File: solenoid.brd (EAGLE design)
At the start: 35.6 x 30.5 mm, 40 parts, among them Y1 ECS-80-S-4X

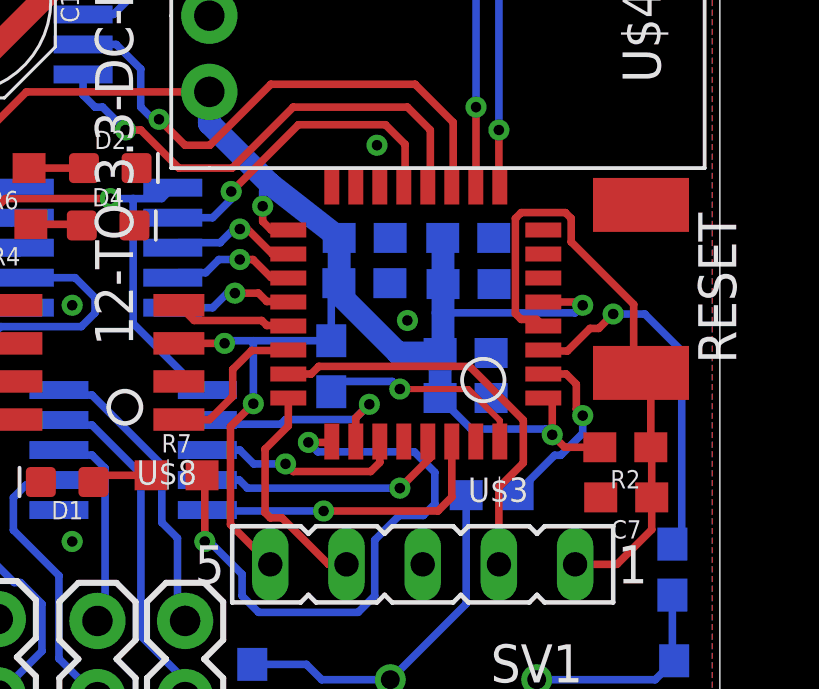
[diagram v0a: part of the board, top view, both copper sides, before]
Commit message: Update solenoid.brd
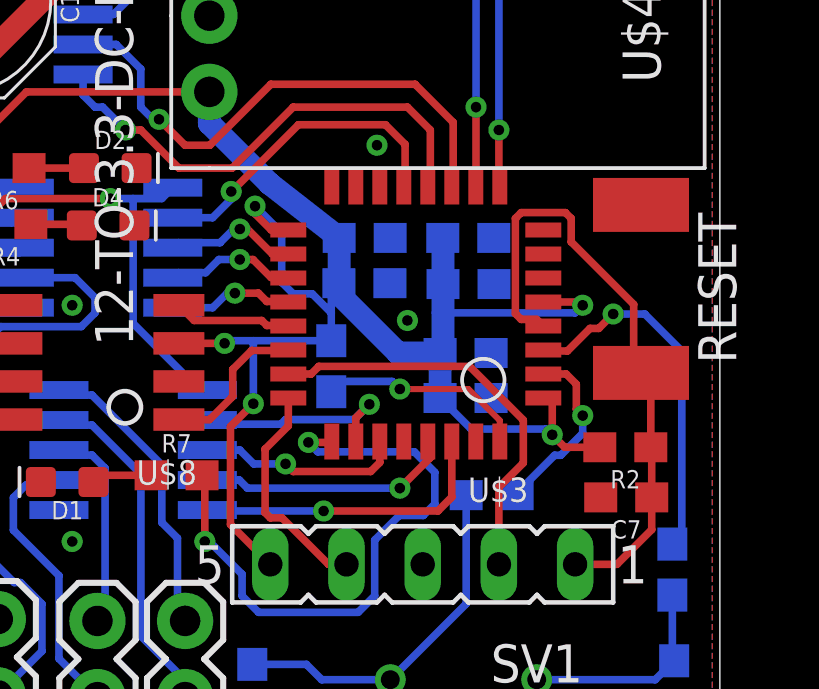
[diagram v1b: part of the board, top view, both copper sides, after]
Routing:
- net +3V3: track 59.1 -> 63.3 mm
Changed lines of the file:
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@@
 <wire x1="29.972" y1="12.148" x2="29.674" y2="12.148" width="0.254" layer="1"/>
 <wire x1="29.972" y1="10.922" x2="29.972" y2="12.148" width="0.254" layer="1"/>
-<wire x1="20.558" y1="19.288" x2="20.32" y2="19.05" width="0.254" layer="16"/>
-<wire x1="20.32" y1="19.05" x2="20.32" y2="18.542" width="0.254" layer="16"/>
-<via x="20.32" y="18.542" extent="1-16" drill="0.35"/>
-<wire x1="20.32" y1="18.542" x2="20.32" y2="18.034" width="0.254" layer="1"/>
-<wire x1="20.32" y1="18.034" x2="20.606" y2="17.748" width="0.254" layer="1"/>
+<via x="20.066" y="18.542" extent="1-16" drill="0.35"/>
+<wire x1="20.066" y1="18.542" x2="20.066" y2="18.288" width="0.254" layer="1"/>
+<wire x1="20.066" y1="18.288" x2="20.606" y2="17.748" width="0.254" layer="1"/>
 <wire x1="20.606" y1="17.748" x2="21.174" y2="17.748" width="0.254" layer="1"/>
 <wire x1="31.558" y1="10.506" x2="30.388" y2="10.506" width="0.254" layer="1"/>
@@
 <via x="20.0084" y="11.95728125" extent="1-16" drill="0.35"/>
 <wire x1="22.86" y1="15.976" x2="22.606" y2="15.722" width="0.254" layer="16"/>
-<wire x1="22.606" y1="15.722" x2="22.606" y2="14.058" width="0.254" layer="16"/>
+<wire x1="22.606" y1="15.722" x2="22.606" y2="14.986" width="0.254" layer="16"/>
+<wire x1="22.606" y1="14.058" x2="22.606" y2="14.986" width="0.254" layer="16"/>
 <wire x1="22.606" y1="14.058" x2="20.0084" y2="14.058" width="0.254" layer="16"/>
 <wire x1="20.0084" y1="14.058" x2="19.138" y2="14.058" width="0.254" layer="16"/>
@@
 <wire x1="10.834" y1="20.74" x2="12.446" y2="22.352" width="0.254" layer="1"/>
 <wire x1="12.446" y1="22.352" x2="18.542" y2="22.352" width="0.254" layer="1"/>
+<wire x1="22.606" y1="14.986" x2="21.971" y2="15.621" width="0.254" layer="16"/>
+<wire x1="21.971" y1="15.621" x2="21.336" y2="15.621" width="0.254" layer="16"/>
+<wire x1="21.336" y1="15.621" x2="20.955" y2="16.002" width="0.254" layer="16"/>
+<wire x1="20.955" y1="16.002" x2="20.955" y2="17.653" width="0.254" layer="16"/>
+<wire x1="20.955" y1="17.653" x2="20.066" y2="18.542" width="0.254" layer="16"/>
 </signal>
 <signal name="GPIO1">
@@
 <wire x1="33.258" y1="10.506" x2="33.288" y2="10.476" width="0.254" layer="1"/>
 <wire x1="33.288" y1="10.476" x2="33.288" y2="8.836" width="0.254" layer="1"/>
-<wire x1="33.288" y1="8.836" x2="33.288" y2="8.58286875" width="0.254" layer="1"/>
 <wire x1="32.931" y1="12.984" x2="33.258" y2="12.657" width="0.254" layer="1"/>
 <wire x1="33.258" y1="12.657" x2="33.258" y2="10.506" width="0.254" layer="1"/>
@@
 <wire x1="32.687" y1="15.2689125" x2="32.687" y2="12.984" width="0.254" layer="1"/>
 <wire x1="30.734" y1="6.604" x2="32.131" y2="6.604" width="0.254" layer="1"/>
+<wire x1="32.131" y1="6.604" x2="33.288" y2="7.761" width="0.254" layer="1"/>
 <wire x1="33.288" y1="7.761" x2="33.288" y2="8.836" width="0.254" layer="1"/>
-<wire x1="32.131" y1="6.604" x2="33.288" y2="7.761" width="0.254" layer="1"/>
 </signal>
 <signal name="SWDIO">
